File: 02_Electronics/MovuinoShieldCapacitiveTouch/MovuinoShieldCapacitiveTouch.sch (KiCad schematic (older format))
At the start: 10 parts, among them J1 DF12_3.0_-36DP_Female, J2 DF12_3.0_-36DP_Male, J3 FH12-10S-0.5SH(55), J4 Conn_01x06_Male, U1 FT5316DME

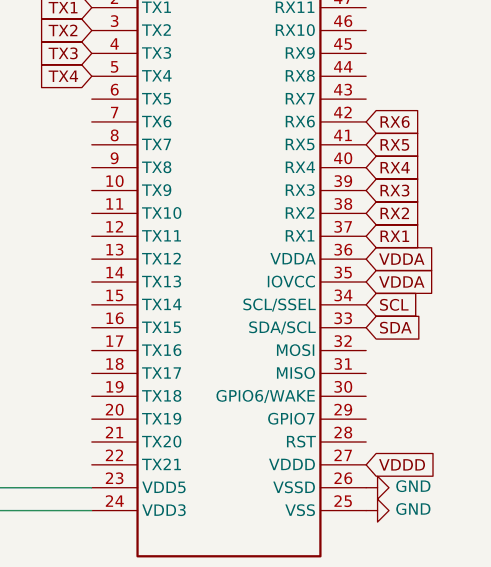
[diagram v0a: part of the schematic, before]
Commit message: shield_v2 done
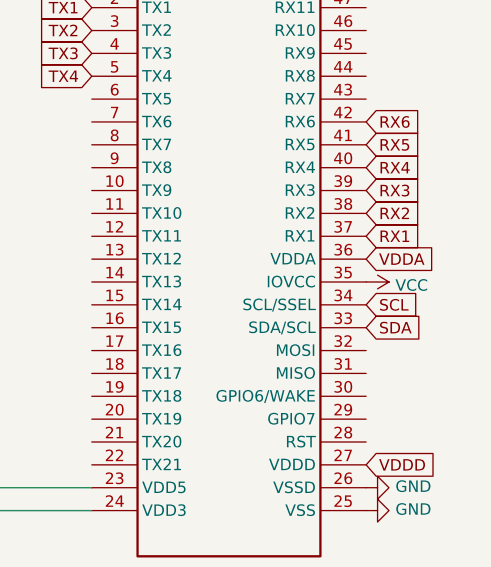
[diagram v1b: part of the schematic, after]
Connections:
- net VCC: now also U1.35 (IOVCC)
- net VDDA: no longer U1.35 (IOVCC)
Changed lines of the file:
@@
 Text GLabel 9400 4000 2    50   Input ~ 0
-VDDA
-Text GLabel 9400 4100 2    50   Input ~ 0
 VDDA
 $Comp
@@
 	0    1    1    0
 $EndComp
+$Comp
+L power:VCC #PWR?
+U 1 1 6254F966
+P 9400 4100
+F 0 "#PWR?" H 9400 3950 50  0001 C CNN
+F 1 "VCC" V 9415 4228 50  0000 L CNN
+F 2 "" H 9400 4100 50  0001 C CNN
+F 3 "" H 9400 4100 50  0001 C CNN
+	1    9400 4100
+	0    1    1    0
+$EndComp
